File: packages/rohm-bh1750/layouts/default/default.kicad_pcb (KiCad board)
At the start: 2 copper layers, 6 parts

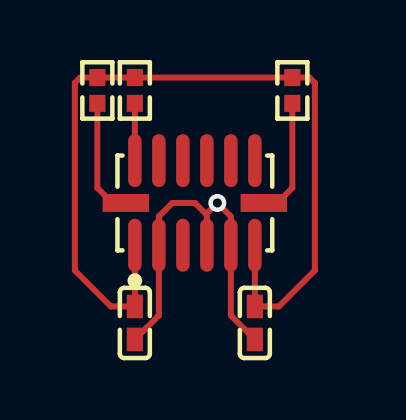
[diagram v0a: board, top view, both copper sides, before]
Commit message: rohm-bh1750: create, rebuild scd40 and bh1750 packages with hide_designators
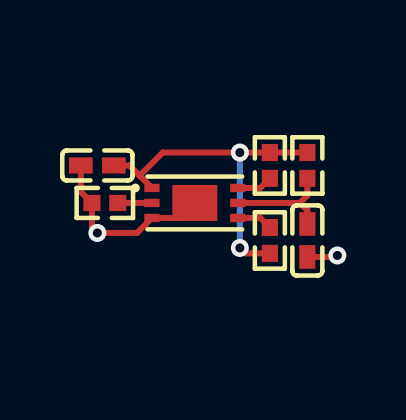
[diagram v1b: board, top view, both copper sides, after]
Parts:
- added R4: 10kΩ ±1% 62.5mW, UNI_ROYAL_0402WGF1002TCE:R0402, F.Cu at (2.50, 1.25)
- R1: value 10kΩ ±1% 62.5mW -> 1kΩ ±1% 62.5mW; footprint UNI_ROYAL_0402WGF1002TCE:R0402 -> UNI_ROYAL_0402WGF1001TCE:R0402
- U1: footprint Analog_Devices_ADXL375BCCZ_RL7:LGA-14_L5.0-W3.0-P0.80-BL -> ROHM_Semicon_BH1750FVI_TR:WSOF-6_L2.6-W1.6-P0.50-TL-EP
- moved C1 7.42 mm to (-3.25, -1.25), turned to 180 degrees
- moved C2 6.37 mm to (3.75, 1.25)
- moved R3 5.15 mm to (2.50, -1.25)
- moved R2 3.76 mm to (-3.00, 0.00), turned to 0 degrees
- moved R1 2.55 mm to (3.75, -1.25), turned to -90 degrees
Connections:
- C1 pad 1: hv -> VCC
- C1 pad 2: -gnd -> gnd
- C2 pad 1: hv -> DVI
- C2 pad 2: -gnd -> gnd
- R1 pad 1: nCS -> VCC
- R1 pad 2: hv -> DVI
- R2 pad 1: SCL_SCLK -> gnd
- R2 pad 2: hv -> ADDR
- R3 pad 1: SDA_SDI_SDIO -> SCL
- R3 pad 2: hv -> VCC
- U1 pad 1: hv -> VCC
- U1 pad 2: -gnd -> ADDR
- U1 pad 3: RESERVED -> gnd
- U1 pad 4: -gnd -> SDA
- U1 pad 5: -gnd -> DVI
- U1 pad 6: hv -> SCL
- U1 pad 7: nCS -> gnd
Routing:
- net hv: track 29.7 -> 0.00 mm
- net -gnd: track 13.0 -> 0.00 mm, vias 1 -> 0
- net VCC: track 0.00 -> 11.7 mm, vias 0 -> 2
- net gnd: track 0.00 -> 7.16 mm, vias 0 -> 2
- net nCS: track 3.98 -> 0.00 mm
- net SCL_SCLK: track 3.98 -> 0.00 mm
- net DVI: track 0.00 -> 3.80 mm
- net SDA_SDI_SDIO: track 1.91 -> 0.00 mm
- net SDA: track 0.00 -> 1.20 mm
- net SCL: track 0.00 -> 1.20 mm
- net ADDR: track 0.00 -> 1.14 mm
